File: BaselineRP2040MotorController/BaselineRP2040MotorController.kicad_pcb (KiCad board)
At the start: 2 copper layers, 88.5 x 63.2 mm, 143 parts, among them J2 Encoder 1, J3 3 Pin XT30 / XT60, J4 XT60 Power Connector, J5 Conn_02x08_Odd_Even, Q1 Q_PNP_BEC, Q2 Q_PNP_BEC, Q3 Q_PNP_BEC, U10 INA240A1D, U11 USBLC6-4SC6, U13 TX4139, U5 EG3113, U6 INA240A1D, U7 EG3113, U8 INA240A1D, U9 EG3113

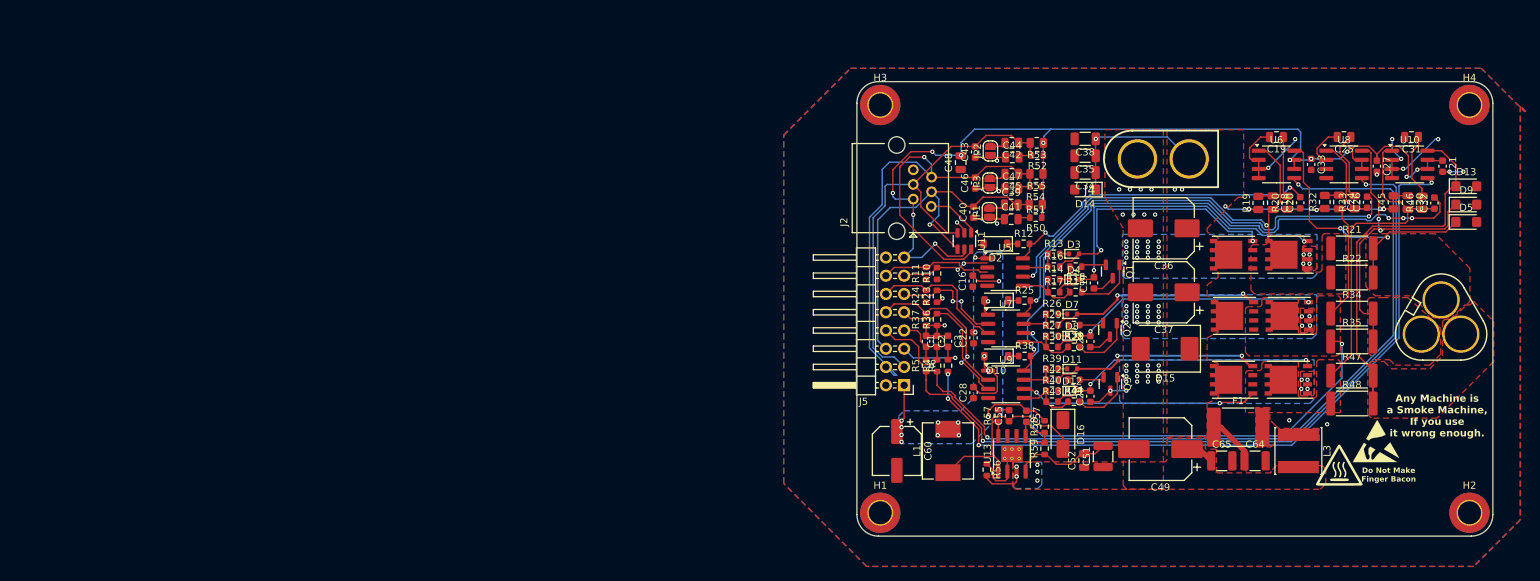
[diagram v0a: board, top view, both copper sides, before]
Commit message: MinMax
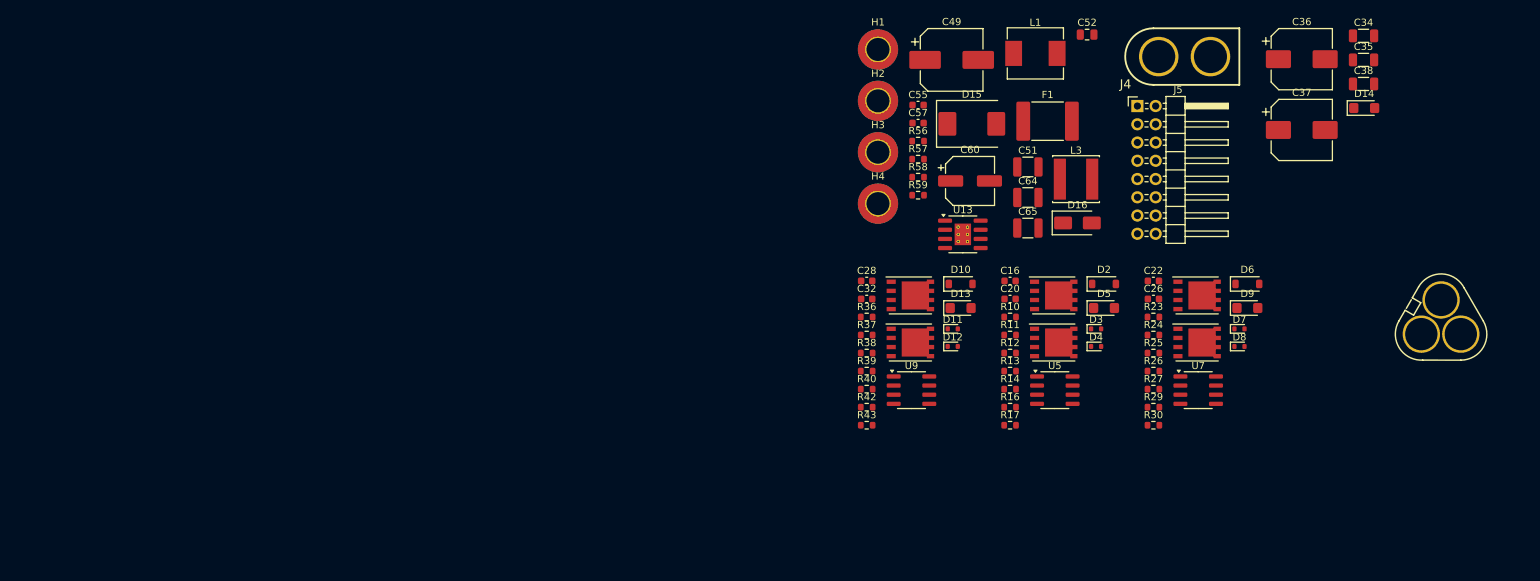
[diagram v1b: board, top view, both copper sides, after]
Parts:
- removed C1, C2, C3: 0, Capacitor_SMD:C_0603_1608Metric
- removed C17, C23, C29: DNP, Capacitor_SMD:C_0603_1608Metric
- removed C18, C19, C24, C25, C30, C31: C, Capacitor_SMD:C_0805_2012Metric
- removed C21, C27, C33: 100n, Capacitor_SMD:C_0603_1608Metric
- removed C39, C42, C45: 22nF, Capacitor_SMD:C_0805_2012Metric
- removed C40, C43, C46: 47p, Capacitor_SMD:C_0603_1608Metric
- removed C41, C44, C47: ~, Capacitor_SMD:C_0805_2012Metric
- removed C48: 10u, Capacitor_SMD:C_0805_2012Metric
- removed J2: Encoder 1, [EastMakes] Connectors:RJ14_Connfly_DS1133-S6_Horizontal
- removed JP1, JP2, JP3: SolderJumper_2_Open, Jumper:SolderJumper-2_P1.3mm_Open_RoundedPad1.0x1.5mm
- removed Q1, Q2, Q3: Q_PNP_BEC, Package_TO_SOT_SMD:SOT-23
- removed R15, R28, R41: 100R, Resistor_SMD:R_0603_1608Metric
- removed R18, R31, R44: 10.2R, Resistor_SMD:R_0603_1608Metric
- removed R19, R20, R32, R33, R45, R46: R, Resistor_SMD:R_0805_2012Metric
- removed R21, R22, R34, R35, R47, R48: 3mΩ, Resistor_SMD:R_2512_6332Metric
- removed R4, R5, R6: 0, Resistor_SMD:R_0603_1608Metric
- removed R50, R52, R54: 10k, Resistor_SMD:R_0603_1608Metric
- removed R51, R53, R55: ~, Resistor_SMD:R_0805_2012Metric
- removed REF**: ESD-Logo_6.6x6mm_SilkScreen, Symbol:ESD-Logo_6.6x6mm_SilkScreen
- removed U10, U6, U8: INA240A1D, Package_SO:SOIC-8_3.9x4.9mm_P1.27mm
- removed U11: USBLC6-4SC6, Package_TO_SOT_SMD:SOT-23-6
- moved H2 100.3 mm to (153.6, 46.3)
- moved H4 83.5 mm to (153.6, 60.6)
- moved C32 80.1 mm to (152.0, 73.8), turned to 0 degrees
- moved D13 72.4 mm to (165.1, 75.1)
- moved H1 64.5 mm to (153.6, 39.1)
- moved C49 61.5 mm to (163.8, 40.6), turned to 0 degrees
- moved C52 59.3 mm to (182.7, 37.1), turned to 0 degrees
- moved L1 56.6 mm to (175.5, 39.7), turned to 0 degrees
- moved AL3 52.8 mm to (158.1, 79.9), turned to 0 degrees
- moved D5 51.8 mm to (185.0, 75.1)
- moved J5 50.6 mm to (189.7, 47.0), turned to 0 degrees
- moved F1 50.2 mm to (177.2, 49.1)
- moved L3 48.9 mm to (181.1, 57.2), turned to 0 degrees
- moved C64 48.4 mm to (174.4, 59.7)
- moved R56 46.7 mm to (159.2, 51.9), turned to 0 degrees
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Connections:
- AH1 pad 1: /BLDC Power Control/Motor Phase U/A_P -> /BLDC Power Control/Motor Phase U/U_OUT
- AH2 pad 1: /BLDC Power Control/Motor Phase V/A_P -> /BLDC Power Control/Motor Phase V/V_OUT
- AH3 pad 1: /BLDC Power Control/Motor Phase X/A_P -> /BLDC Power Control/Motor Phase X/X_OUT
- AL1 pad 3: /BLDC Power Control/Motor Phase U/A_P -> /BLDC Power Control/Motor Phase U/U_OUT
- AL2 pad 3: /BLDC Power Control/Motor Phase V/A_P -> /BLDC Power Control/Motor Phase V/V_OUT
- AL3 pad 3: /BLDC Power Control/Motor Phase X/A_P -> /BLDC Power Control/Motor Phase X/X_OUT
- C20 pad 1: /BLDC Power Control/Motor Phase U/A_P -> /BLDC Power Control/Motor Phase U/U_OUT
- C26 pad 1: /BLDC Power Control/Motor Phase V/A_P -> /BLDC Power Control/Motor Phase V/V_OUT
- C32 pad 1: /BLDC Power Control/Motor Phase X/A_P -> /BLDC Power Control/Motor Phase X/X_OUT
- D13 pad 1: /BLDC Power Control/Motor Phase X/A_N -> /BLDC Power Control/Motor Phase X/X_OUT
- D5 pad 1: /BLDC Power Control/Motor Phase U/A_N -> /BLDC Power Control/Motor Phase U/U_OUT
- D9 pad 1: /BLDC Power Control/Motor Phase V/A_N -> /BLDC Power Control/Motor Phase V/V_OUT
- J3 pad 1: /BLDC Power Control/Motor Phase U/A_N -> /BLDC Power Control/Motor Phase U/U_OUT
- J3 pad 2: /BLDC Power Control/Motor Phase V/A_N -> /BLDC Power Control/Motor Phase V/V_OUT
- J3 pad 3: /BLDC Power Control/Motor Phase X/A_N -> /BLDC Power Control/Motor Phase X/X_OUT
- J5 pad 15: +3V3 -> /3V3
- U5 pad 6: /BLDC Power Control/Motor Phase U/A_P -> /BLDC Power Control/Motor Phase U/U_OUT
- U7 pad 6: /BLDC Power Control/Motor Phase V/A_P -> /BLDC Power Control/Motor Phase V/V_OUT
- U9 pad 6: /BLDC Power Control/Motor Phase X/A_P -> /BLDC Power Control/Motor Phase X/X_OUT
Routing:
- net +3V3: track 142.3 -> 0.00 mm, vias 11 -> 0
- net Net-(R4-Pad1): track 110.0 -> 0.00 mm, vias 2 -> 0
- net Net-(R5-Pad1): track 104.7 -> 0.00 mm, vias 2 -> 0
- net Net-(R6-Pad1): track 103.4 -> 0.00 mm, vias 4 -> 0
- net GND: track 99.9 -> 0.00 mm, vias 87 -> 0
- net /BLDC Power Control/Motor Phase V/A_P: track 99.0 -> 0.00 mm, vias 2 -> 0
- net /Encoder SCK: track 86.4 -> 0.00 mm, vias 1 -> 0
- net Net-(U9-VB): track 83.1 -> 0.00 mm, vias 4 -> 0
- net /BLDC Power Control/Motor Phase X/A_P: track 79.9 -> 0.00 mm, vias 2 -> 0
- net /Encoder CS: track 65.9 -> 0.00 mm
- net Net-(U7-VB): track 65.7 -> 0.00 mm, vias 2 -> 0
- net /BLDC Power Control/Motor Phase U/A_P: track 59.7 -> 0.00 mm, vias 2 -> 0
- net /Encoder RX: track 57.3 -> 0.00 mm, vias 1 -> 0
- net VMOT_PWR: track 56.0 -> 0.00 mm, vias 7 -> 0
- net /BLDC Power Control/Motor Phase X/A_N: track 54.5 -> 0.00 mm
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- removed copper zone on B.Cu, net +12V
- removed copper zone on F.Cu, net /BLDC Power Control/Motor Phase U/A_N
- removed copper zone on F.Cu, net /BLDC Power Control/Motor Phase U/A_P
- removed copper zone on F.Cu, net /BLDC Power Control/Motor Phase V/A_N
- removed copper zone on F.Cu, net /BLDC Power Control/Motor Phase V/A_P
- removed copper zone on F.Cu, net /BLDC Power Control/Motor Phase X/A_N
- removed copper zone on F.Cu, net /BLDC Power Control/Motor Phase X/A_P
- removed copper zone on B.Cu, net GND
- removed copper zone on F.Cu, net GND
- removed copper zone on F.Cu, net Net-(F1-Pad2)
- removed copper zone on B.Cu, net VMOT
- removed copper zone on F.Cu, net VMOT
- removed copper zone on F.Cu, net VMOT_PWR
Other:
- board outline removed
- board text removed: "Any Machine is a Smoke Machine, If you use it wrong enough."
- board text removed: "Do Not Make Finger Bacon"

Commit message: Heh - Super cut down.
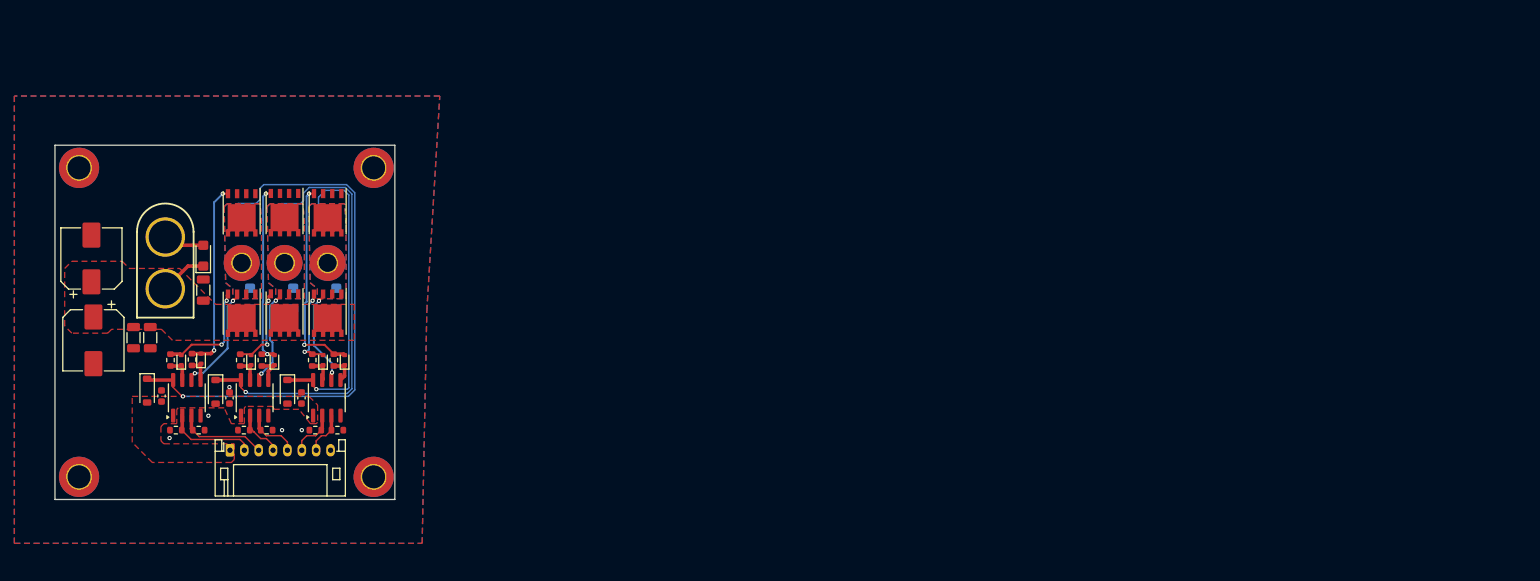
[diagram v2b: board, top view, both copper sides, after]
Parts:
- removed C49: 47uF 63V solid, Capacitor_SMD:CP_Elec_8x10.5
- removed C51, C64, C65: 4.7uF 100V, Capacitor_SMD:C_1210_3225Metric
- removed C52: 100nF 100V, Capacitor_SMD:C_0805_2012Metric
- removed C55: 100n, Capacitor_SMD:C_0603_1608Metric
- removed C57: 47p, Capacitor_SMD:C_0603_1608Metric
- removed C60: 220uF 25V, Capacitor_SMD:CP_Elec_6.3x7.7
- removed D15: SMAJ51A, Diode_SMD:D_SMC
- removed D16: SS310, Diode_SMD:D_SMA
- removed F1: 60V 1.5A hold polyfuse, Fuse:Fuse_2920_7451Metric
- removed J3: 3 Pin XT30 / XT60, [EastMakes] Connectors:MT60-F.G.Y
- removed J5: Conn_02x08_Odd_Even, Connector_PinHeader_2.54mm:PinHeader_2x08_P2.54mm_Horizontal
- removed L1: 47uH, Inductor_SMD:L_Chilisin_BMRB00060612
- removed L3: 68uH 1A, Inductor_SMD:L_Sunlord_SWPA6045S
- removed R12, R13, R14, R25, R26, R27, R38, R39, R40: 0R, Resistor_SMD:R_0603_1608Metric
- removed R56: 30mΩ 5%, Resistor_SMD:R_0603_1608Metric
- removed R57: 10Ω, Resistor_SMD:R_0603_1608Metric
- removed R58: 300k, Resistor_SMD:R_0603_1608Metric
- removed R59: 21.5k, Resistor_SMD:R_0603_1608Metric
- removed U13: TX4139, Package_SO:SOIC-8-1EP_3.9x4.9mm_P1.27mm_EP2.29x3mm_ThermalVias
- added H5: MountingHole_Pad, MountingHole:MountingHole_2.5mm_Pad_TopBottom, F.Cu at (65.0, 68.8)
- added H6: MountingHole_Pad, MountingHole:MountingHole_2.5mm_Pad_TopBottom, F.Cu at (71.0, 68.8)
- added H7: MountingHole_Pad, MountingHole:MountingHole_2.5mm_Pad_TopBottom, F.Cu at (77.0, 68.8)
- added J1: Conn_01x08, Connector_JST:JST_PH_S8B-PH-K_1x08_P2.00mm_Horizontal, F.Cu at (63.4, 94.9)
- C20, C26, C32, D13, D5, D9: moved to B.Cu
- moved C34 176.3 mm to (50.0, 79.2), turned to -90 degrees
- moved C35 173.2 mm to (52.3, 79.2), turned to -90 degrees
- moved C36 170.7 mm to (44.1, 68.2), turned to 90 degrees
- moved C37 170.7 mm to (44.4, 79.6), turned to -90 degrees
- moved C38 164.0 mm to (59.7, 72.6), turned to 90 degrees
- moved D14 162.9 mm to (59.7, 67.8), turned to 90 degrees
- moved J4 144.7 mm to (54.4, 68.8), turned to -90 degrees
- moved D6 144.4 mm to (61.4, 86.8), turned to -90 degrees
- moved D7 137.6 mm to (66.3, 82.3), turned to 90 degrees
- moved D8 134.3 mm to (69.6, 82.3), turned to 90 degrees
- moved D2 134.0 mm to (51.9, 86.6), turned to -90 degrees
- moved D9 132.8 mm to (72.2, 73.8), turned to -90 degrees
- moved U7 131.3 mm to (66.8, 87.6), turned to 90 degrees
- moved C22 129.6 mm to (63.3, 87.6), turned to -90 degrees
- moved AL2 128.3 mm to (71.0, 61.8), turned to -90 degrees
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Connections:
- C20 pad 2: Net-(U5-VB) -> Net-(D2-K)
- C26 pad 2: Net-(U7-VB) -> Net-(D6-K)
- C32 pad 2: Net-(U9-VB) -> Net-(D10-K)
- R16 pad 1: Net-(U5-HO) -> Net-(D3-K)
- R17 pad 1: Net-(U5-LO) -> Net-(D4-K)
- R29 pad 1: Net-(U7-HO) -> Net-(D7-K)
- R30 pad 1: Net-(U7-LO) -> Net-(D8-K)
- R42 pad 1: Net-(U9-HO) -> Net-(D11-K)
- R43 pad 1: Net-(U9-LO) -> Net-(D12-K)
- U5 pad 5: Net-(U5-LO) -> Net-(D4-K)
- U5 pad 7: Net-(U5-HO) -> Net-(D3-K)
- U5 pad 8: Net-(U5-VB) -> Net-(D2-K)
- U7 pad 5: Net-(U7-LO) -> Net-(D8-K)
- U7 pad 7: Net-(U7-HO) -> Net-(D7-K)
- U7 pad 8: Net-(U7-VB) -> Net-(D6-K)
- U9 pad 5: Net-(U9-LO) -> Net-(D12-K)
- U9 pad 7: Net-(U9-HO) -> Net-(D11-K)
- U9 pad 8: Net-(U9-VB) -> Net-(D10-K)
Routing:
- net Net-(D2-K): track 0.00 -> 78.2 mm, vias 0 -> 1
- net Net-(D6-K): track 0.00 -> 60.6 mm, vias 0 -> 1
- net Net-(D10-K): track 0.00 -> 43.0 mm, vias 0 -> 1
- net Net-(AL3-G): track 0.00 -> 28.5 mm, vias 0 -> 2
- net Net-(AL1-G): track 0.00 -> 26.5 mm, vias 0 -> 2
- net Net-(AL2-G): track 0.00 -> 25.3 mm, vias 0 -> 2
- net /BLDC Power Control/Motor Phase U/U_OUT: track 0.00 -> 15.2 mm, vias 0 -> 2
- net Net-(AH1-G): track 0.00 -> 15.2 mm, vias 0 -> 2
- net /BLDC Power Control/Motor Phase V/V_OUT: track 0.00 -> 12.5 mm, vias 0 -> 2
- net /BLDC Power Control/Motor Phase X/X_OUT: track 0.00 -> 12.5 mm, vias 0 -> 2
- net /PWM H U: track 0.00 -> 12.4 mm
- net /PWM L U: track 0.00 -> 12.4 mm
- net Net-(AH2-G): track 0.00 -> 11.8 mm, vias 0 -> 2
- net Net-(AH3-G): track 0.00 -> 11.5 mm, vias 0 -> 2
- net /PWM L V: track 0.00 -> 7.66 mm
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- added copper zone on F.Cu, net +12V
- added copper zone on B.Cu, net /BLDC Power Control/Motor Phase U/U_OUT
- added copper zone on F.Cu, net /BLDC Power Control/Motor Phase U/U_OUT
- added copper zone on B.Cu, net /BLDC Power Control/Motor Phase V/V_OUT
- added copper zone on F.Cu, net /BLDC Power Control/Motor Phase V/V_OUT
- added copper zone on B.Cu, net /BLDC Power Control/Motor Phase X/X_OUT
- added copper zone on F.Cu, net /BLDC Power Control/Motor Phase X/X_OUT
- added copper zone on B.Cu, net GND
- added copper zone on F.Cu, net GND
- added copper zone on F.Cu, net VMOT_PWR
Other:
- board outline added: 47.3 x 49.3 mm
